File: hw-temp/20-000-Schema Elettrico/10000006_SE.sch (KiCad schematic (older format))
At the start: 38 parts, among them P1 PLUG_01X04_254, P2 PLUG_01X04_254, P3 PLUG_01X04_254, P4 PLUG_01X04_254, P5 PLUG_01X04_254, P6 PLUG_01X04_254, P7 PLUG_01X04_254, P8 PLUG_01X04_254, U1 TPS709, U2 PCA9306DC, U3 SC18IS602BIPW, U4 MAX31865

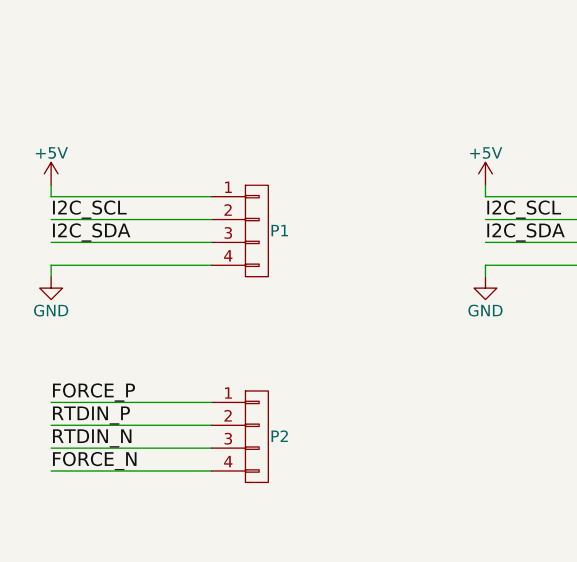
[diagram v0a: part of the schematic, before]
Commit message: PCB terminato
Signed-off-by: CrazyDiamond <crazyd14@gmail.com>
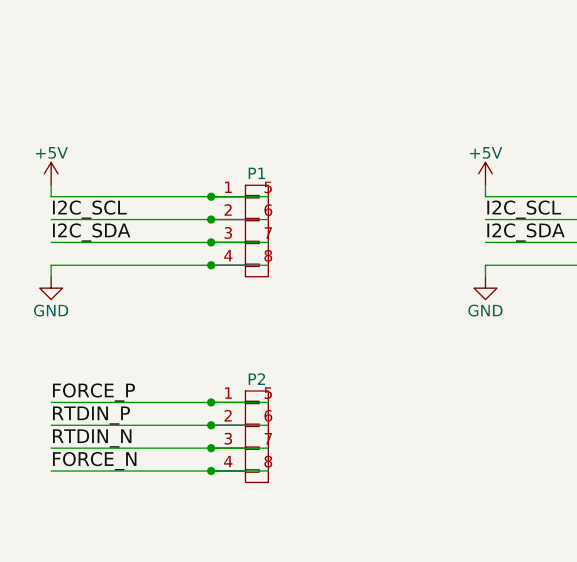
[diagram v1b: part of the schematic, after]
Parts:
- removed P1, P2: PLUG_01X04_254, Socket_Strips:Socket_Strip_Straight_1x04, symbol PLUG_01X04_254
- added P1, P2: TERMINAL_01X04_250_RA_SPRING, os_terminal_block:1770908, symbol TERMINAL_01X04_250_RA_SPRING
